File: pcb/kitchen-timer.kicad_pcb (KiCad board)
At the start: 2 copper layers, 41 x 33 mm, 23 parts, among them IC1 ArduinoProMini, J1 EX, J2 3.3V, J3 RT, J4 Conn_01x03, J5 Conn_01x03, J6 LCD, Q1 BC337, Q2 BC327, Q3 BC337, Q4 BC327, Q5 BC337

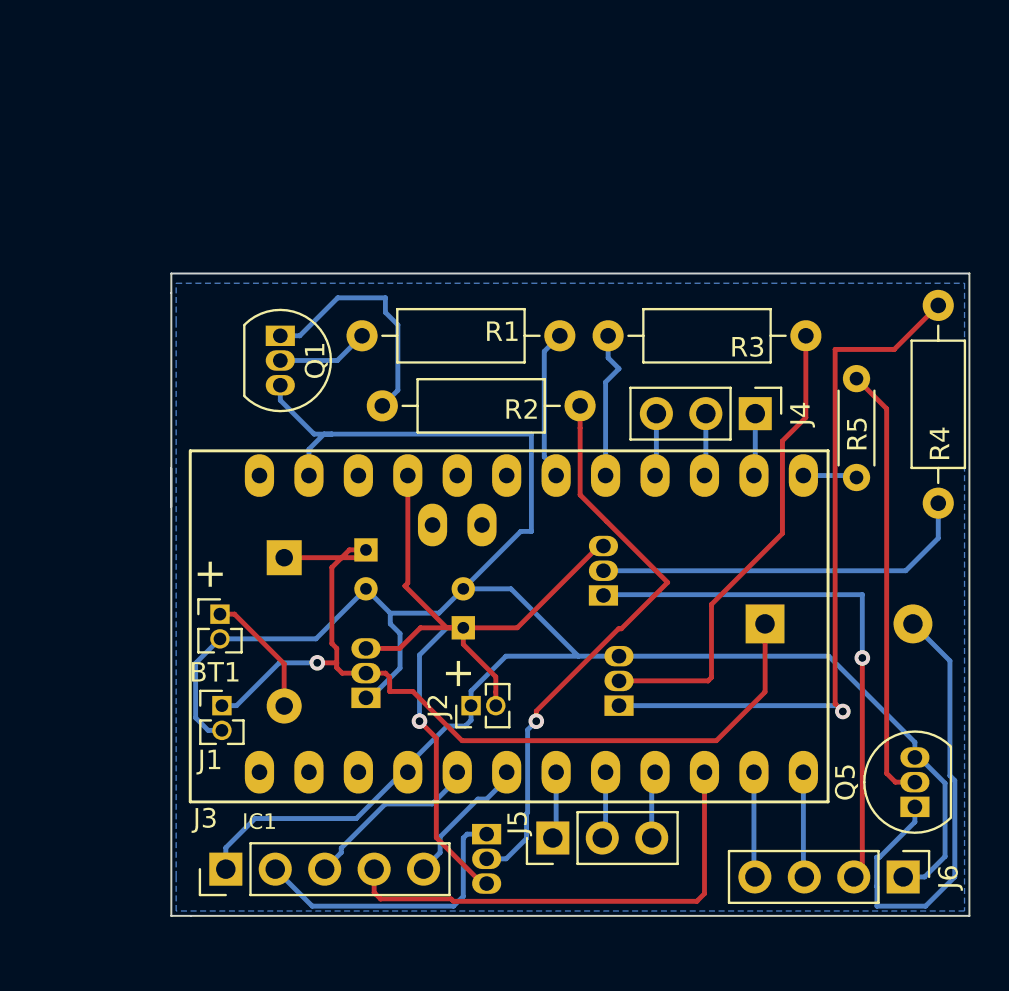
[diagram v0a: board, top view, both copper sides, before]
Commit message: add pcb
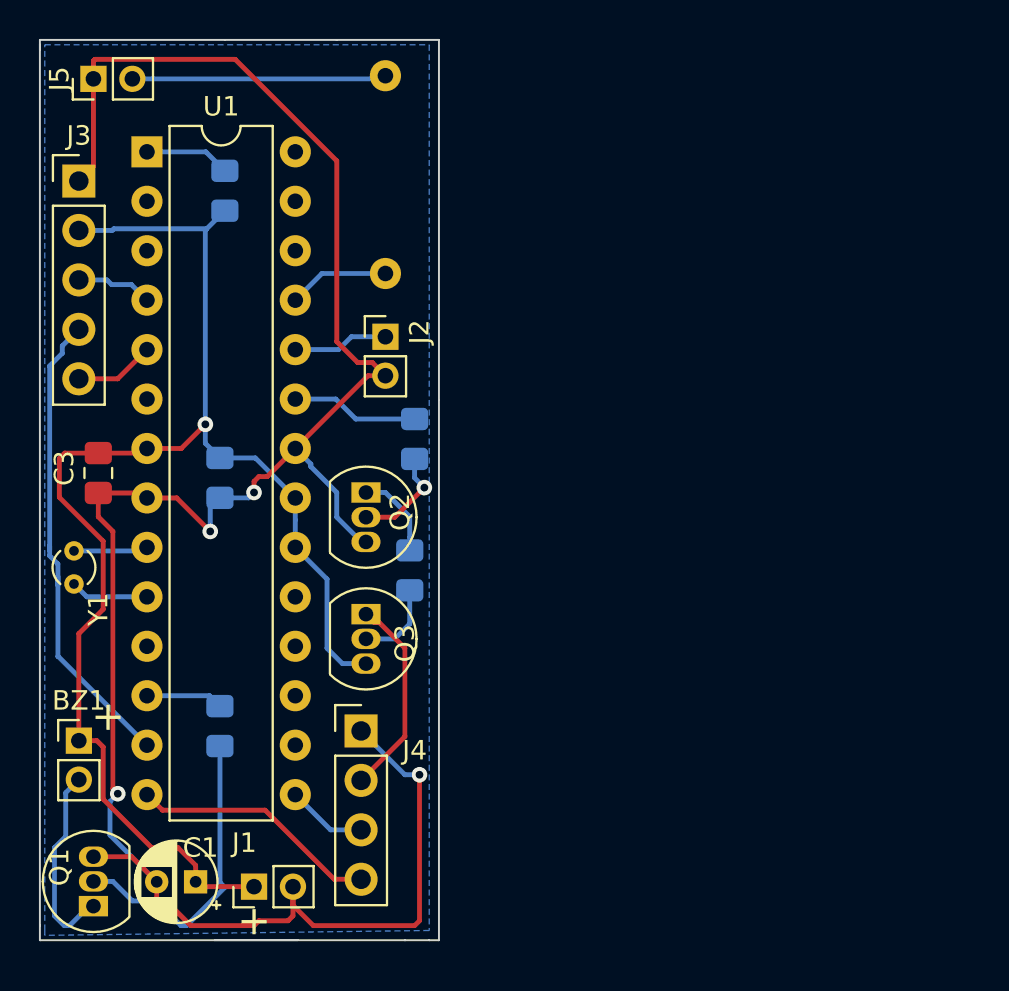
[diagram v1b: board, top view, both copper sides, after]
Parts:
- removed BT1: 9V, Connector_PinHeader_1.27mm:PinHeader_1x02_P1.27mm_Vertical
- removed D1: D, Diode_THT:D_A-405_P7.62mm_Horizontal
- removed IC1: ArduinoProMini, arduino:pro_mini
- removed J6: LCD, Connector_PinHeader_2.54mm:PinHeader_1x04_P2.54mm_Vertical
- removed L1: HT7333-A, Package_TO_SOT_THT:TO-92_Inline
- removed Q4: BC327, Package_TO_SOT_THT:TO-92_Inline
- removed Q5: BC337, Package_TO_SOT_THT:TO-92_Inline
- added C3: 100nf, Capacitor_SMD:C_0805_2012Metric_Pad1.15x1.40mm_HandSolder, F.Cu at (109.2, 82.2)
- added U1: ATmega328-PU, Package_DIP:DIP-28_W7.62mm, F.Cu at (111.8, 65.8)
- added Y1: 32khz, Crystal:Crystal_DS15_D1.5mm_L5.0mm_Vertical, F.Cu at (108.0, 86.2)
- BZ1: footprint Buzzer_Beeper:Buzzer_12x9.5RM7.6 -> Connector_PinHeader_2.00mm:PinHeader_1x02_P2.00mm_Vertical; moved to F.Cu
- C1: moved to F.Cu
- C2: value 10uF -> 100nf; footprint Capacitor_THT:CP_Radial_D4.0mm_P2.00mm -> Capacitor_SMD:C_0805_2012Metric_Pad1.15x1.40mm_HandSolder
- J1: value EX -> USB_Breakout IN; footprint Connector_PinHeader_1.27mm:PinHeader_1x02_P1.27mm_Vertical -> Connector_PinHeader_2.00mm:PinHeader_1x02_P2.00mm_Vertical
- J2: value 3.3V -> SW2; footprint Connector_PinHeader_1.27mm:PinHeader_1x02_P1.27mm_Vertical -> Connector_PinHeader_2.00mm:PinHeader_1x02_P2.00mm_Vertical
- J4: value Conn_01x03 -> LCD; footprint Connector_PinHeader_2.54mm:PinHeader_1x03_P2.54mm_Vertical -> Connector_PinHeader_2.54mm:PinHeader_1x04_P2.54mm_Vertical
- J5: value Conn_01x03 -> LED1; footprint Connector_PinHeader_2.54mm:PinHeader_1x03_P2.54mm_Vertical -> Connector_PinHeader_2.00mm:PinHeader_1x02_P2.00mm_Vertical
- Q2: value BC327 -> BC337; moved to F.Cu
- Q3: value BC337 -> BC327; moved to F.Cu
- R1: value 2.6k -> 10k; footprint Resistor_THT:R_Axial_DIN0207_L6.3mm_D2.5mm_P10.16mm_Horizontal -> Resistor_SMD:R_0805_2012Metric_Pad1.15x1.40mm_HandSolder; moved to B.Cu
- R2, R3, R4: footprint Resistor_THT:R_Axial_DIN0207_L6.3mm_D2.5mm_P10.16mm_Horizontal -> Resistor_SMD:R_0805_2012Metric_Pad1.15x1.40mm_HandSolder; moved to B.Cu
- R5: value 2.6k -> 220; footprint Resistor_THT:R_Axial_DIN0204_L3.6mm_D1.6mm_P5.08mm_Horizontal -> Resistor_THT:R_Axial_DIN0207_L6.3mm_D2.5mm_P10.16mm_Horizontal; moved to B.Cu
- moved J5 45.6 mm to (109.0, 62.0)
- moved J3 36.1 mm to (108.2, 67.2), turned to 0 degrees
- moved BZ1 35.8 mm to (108.2, 96.0)
- moved Q1 30.8 mm to (109.0, 104.5), turned to 90 degrees
- moved R4 27.4 mm to (125.2, 87.2)
- moved J4 26.0 mm to (122.8, 95.5), turned to 0 degrees
- moved R5 24.8 mm to (124.0, 72.0), turned to 90 degrees
- moved R2 24.8 mm to (115.5, 95.2), turned to 90 degrees
- moved R3 20.8 mm to (125.5, 80.5), turned to 90 degrees
- moved J2 19.5 mm to (124.0, 75.2), turned to 0 degrees
- moved C1 19.2 mm to (114.2, 103.2), turned to 180 degrees
- moved Q2 18.6 mm to (123.0, 83.2)
- moved C2 14.7 mm to (115.5, 82.5), turned to 270 degrees
- moved Q3 13.8 mm to (123.0, 89.5), turned to 270 degrees
- moved R1 10.3 mm to (115.8, 67.8), turned to 90 degrees
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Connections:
- BZ1 pad 1: Net-(BZ1-Pad1) -> +3V3
- C1 pad 1: Net-(BZ1-Pad1) -> +3V3
- C1 pad 2: -BATT -> GND
- C2 pad 2: -BATT -> GND
- J1 pad 1: Net-(BZ1-Pad1) -> +3V3
- J1 pad 2: -BATT -> GND
- J2 pad 1: -BATT -> Net-(J2-Pad1)
- J2 pad 2: +3V3 -> GND
- J3 pad 1: -BATT -> GND
- J3 pad 2: Net-(J3-Pad2) -> +3V3
- J4 pad 1: Net-(IC1-Pad14) -> GND
- J4 pad 2: Net-(IC1-Pad15) -> Net-(J4-Pad2)
- J4 pad 3: Net-(IC1-Pad16) -> LCD_DIO
- J5 pad 1: Net-(IC1-Pad7) -> GND
- J5 pad 2: Net-(IC1-Pad8) -> Net-(J5-Pad2)
- Q1 pad 1: Net-(Q1-Pad1) -> Net-(BZ1-Pad2)
- Q1 pad 3: -BATT -> GND
- Q2 pad 1: Net-(J3-Pad2) -> Net-(Q2-Pad1)
- Q2 pad 3: +3V3 -> GND
- Q3 pad 1: Net-(Q3-Pad1) -> Net-(J4-Pad2)
- Q3 pad 3: -BATT -> +3V3
- R1 pad 1: Net-(Q1-Pad2) -> +3V3
- R1 pad 2: ENABLE_RT -> Net-(R1-Pad2)
- R2 pad 1: Net-(Q2-Pad2) -> Net-(Q1-Pad2)
- R2 pad 2: Net-(Q1-Pad1) -> Net-(R2-Pad2)
- R3 pad 1: Net-(Q3-Pad2) -> Net-(Q2-Pad2)
- R4 pad 1: Net-(Q4-Pad2) -> Net-(Q3-Pad2)
- R4 pad 2: Net-(Q3-Pad1) -> Net-(Q2-Pad1)
- R5 pad 2: BUZZER -> Net-(J5-Pad2)
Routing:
- net GND: track 0.00 -> 114.9 mm, vias 0 -> 4
- net -BATT: track 113.2 -> 0.00 mm
- net Net-(BZ1-Pad1): track 47.1 -> 0.00 mm, vias 1 -> 0
- net Net-(Q3-Pad1): track 36.6 -> 0.00 mm, vias 1 -> 0
- net +3V3: track 44.8 -> 73.8 mm
- net Net-(J6-Pad2): track 28.0 -> 0.00 mm, vias 1 -> 0
- net Net-(Q2-Pad2): track 29.7 -> 5.31 mm
- net Net-(Q3-Pad2): track 24.4 -> 4.29 mm
- net Net-(Q4-Pad2): track 19.7 -> 0.00 mm
- net Net-(R5-Pad1): track 22.6 -> 5.20 mm
- net Net-(J3-Pad2): track 14.9 -> 0.00 mm
- net Net-(BZ1-Pad2): track 24.5 -> 10.1 mm
- net Net-(J5-Pad2): track 0.00 -> 13.1 mm
- net Net-(Q1-Pad1): track 12.4 -> 0.00 mm
- net Net-(Q1-Pad2): track 4.73 -> 15.9 mm
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- added copper zone on B.Cu, net GND
- removed copper zone on B.Cu, net -BATT
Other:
- board size 41 x 33 mm -> 20.5 x 46.2 mm
